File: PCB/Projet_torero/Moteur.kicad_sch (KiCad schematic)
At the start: 5 parts, among them J601 Conn_01x06, U601 ZXBM5210-SP

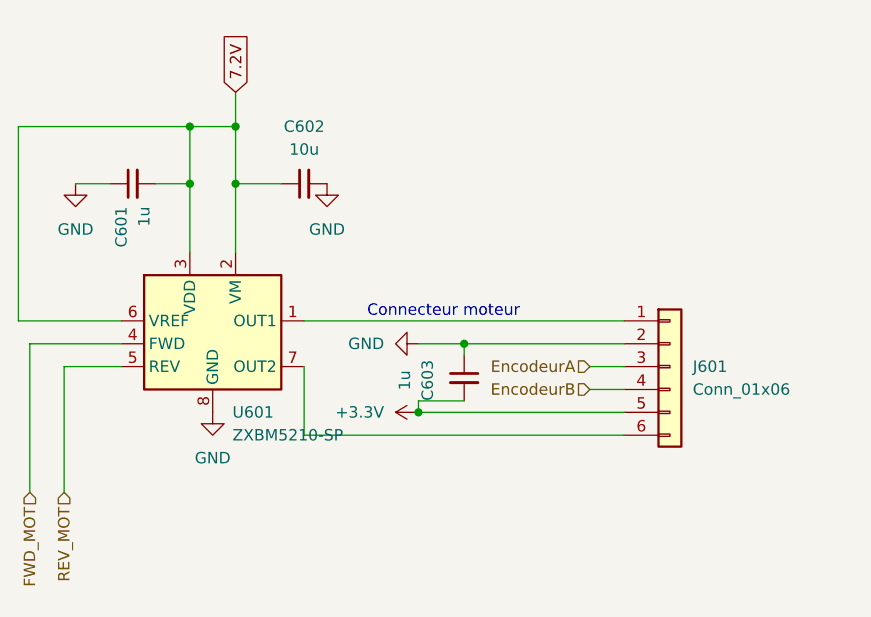
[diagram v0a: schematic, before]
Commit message: Correction suggestion prof
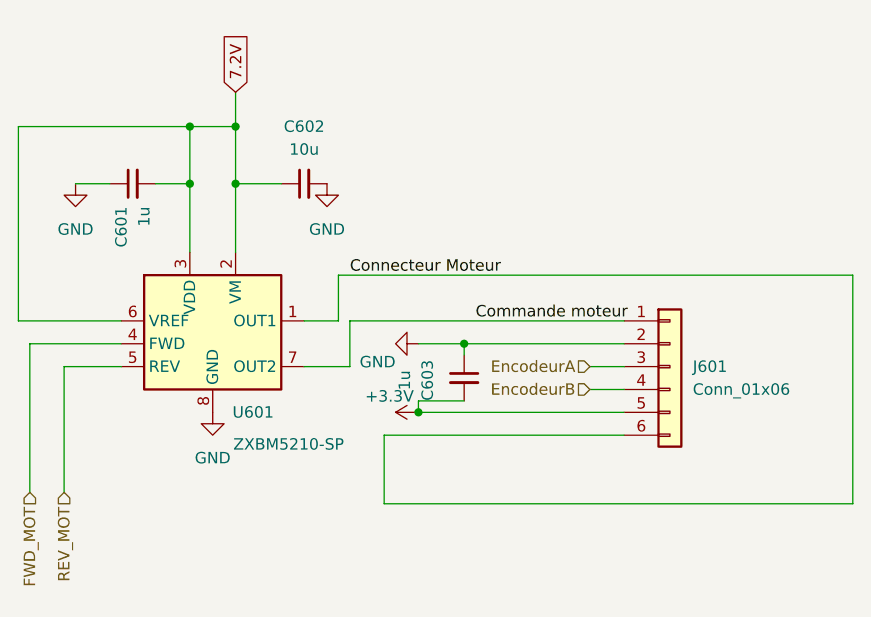
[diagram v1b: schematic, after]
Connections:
- net Commande moteur: now reaches J601.1 (Pin_1)
- net Commande moteur: now also U601.7 (OUT2); no longer U601.1 (OUT1)
- net Connecteur Moteur: now reaches J601.6 (Pin_6)
- net Connecteur Moteur: now also U601.1 (OUT1); no longer U601.7 (OUT2)
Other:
- note removed: "Connecteur moteur"
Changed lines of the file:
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@@
+	(wire
+		(pts
+			(xy 149.86 66.04) (xy 154.94 66.04)
+		)
+		(stroke
+			(width 0)
+			(type default)
+		)
+	)
 	(wire
 		(pts
@@
 	(wire
 		(pts
+			(xy 158.75 73.66) (xy 185.42 73.66)
+		)
+		(stroke
+			(width 0)
+			(type default)
+		)
+	)
+	(wire
+		(pts
 			(xy 181.61 68.58) (xy 185.42 68.58)
 		)
@@
 	(wire
 		(pts
-			(xy 149.86 60.96) (xy 185.42 60.96)
+			(xy 154.94 60.96) (xy 185.42 60.96)
 		)
 		(stroke
@@
 	(wire
 		(pts
+			(xy 210.82 55.88) (xy 210.82 81.28)
+		)
+		(stroke
+			(width 0)
+			(type default)
+		)
+	)
+	(wire
+		(pts
 			(xy 162.56 69.85) (xy 162.56 71.12)
 		)
@@
 	(wire
 		(pts
+			(xy 210.82 81.28) (xy 158.75 81.28)
+		)
+		(stroke
+			(width 0)
+			(type default)
+		)
+	)
+	(wire
+		(pts
+			(xy 153.67 55.88) (xy 210.82 55.88)
+		)
+		(stroke
+			(width 0)
+			(type default)
+		)
+	)
+	(wire
+		(pts
+			(xy 154.94 60.96) (xy 154.94 66.04)
+		)
+		(stroke
+			(width 0)
+			(type default)
+		)
+	)
+	(wire
+		(pts
+			(xy 153.67 55.88) (xy 153.67 60.96)
+		)
+		(stroke
+			(width 0)
+			(type default)
+		)
+	)
+	(wire
+		(pts
+			(xy 158.75 81.28) (xy 158.75 73.66)
+		)
+		(stroke
+			(width 0)
+			(type default)
+		)
+	)
+	(wire
+		(pts
 			(xy 123.19 66.04) (xy 129.54 66.04)
 		)
@@
 	(wire
 		(pts
-			(xy 149.86 73.66) (xy 149.86 66.04)
+			(xy 149.86 60.96) (xy 153.67 60.96)
 		)
 		(stroke
@@
 	(wire
 		(pts
-			(xy 149.86 73.66) (xy 185.42 73.66)
-		)
-		(stroke
-			(width 0)
-			(type default)
-		)
-	)
-	(wire
-		(pts
 			(xy 167.64 63.5) (xy 185.42 63.5)
 		)
@@
 		)
 	)
-	(text "Connecteur moteur"
-		(exclude_from_sim no)
-		(at 165.354 59.944 0)
+	(label "Connecteur Moteur"
+		(at 154.94 55.88 0)
+		(fields_autoplaced yes)
 		(effects
 			(font
 				(size 1.27 1.27)
 			)
+			(justify left bottom)
+		)
+	)
+	(label "Commande moteur"
+		(at 168.91 60.96 0)
+		(fields_autoplaced yes)
+		(effects
+			(font
+				(size 1.27 1.27)
+			)
+			(justify left bottom)
 		)
 	)
@@
 		(on_board yes)
 		(dnp no)
-		(fields_autoplaced yes)
 		(property "Reference" "#PWR0605"
 			(at 166.37 71.12 0)
@@
 		)
 		(property "Value" "+3.3V"
-			(at 158.75 71.1199 90)
+			(at 162.052 69.342 90)
 			(effects
 				(font
@@
 		(on_board yes)
 		(dnp no)
-		(fields_autoplaced yes)
 		(property "Reference" "U601"
 			(at 141.8941 71.12 0)
@@
 		)
 		(property "Value" "ZXBM5210-SP"
-			(at 141.8941 73.66 0)
+			(at 141.986 74.676 0)
 			(effects
 				(font
@@
 		(on_board yes)
 		(dnp no)
-		(fields_autoplaced yes)
 		(property "Reference" "#PWR0604"
 			(at 156.21 63.5 0)
@@
 		)
 		(property "Value" "GND"
-			(at 158.75 63.4999 90)
-			(effects
-				(font
+			(at 160.02 65.532 90)
+			(effects
+				(font
